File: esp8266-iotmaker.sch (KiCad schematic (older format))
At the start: 49 parts, among them J1 CONN_01X10, J2 CONN_01X10, Q1 S8050, Q2 S8050, SW1 SW_Push, SW2 SW_Push, U1 usb_mini_b, U2 chip-esp8266, U3 CP2102, U4 25Q32, U6 AMS1117-3.3, Y1 26MHz

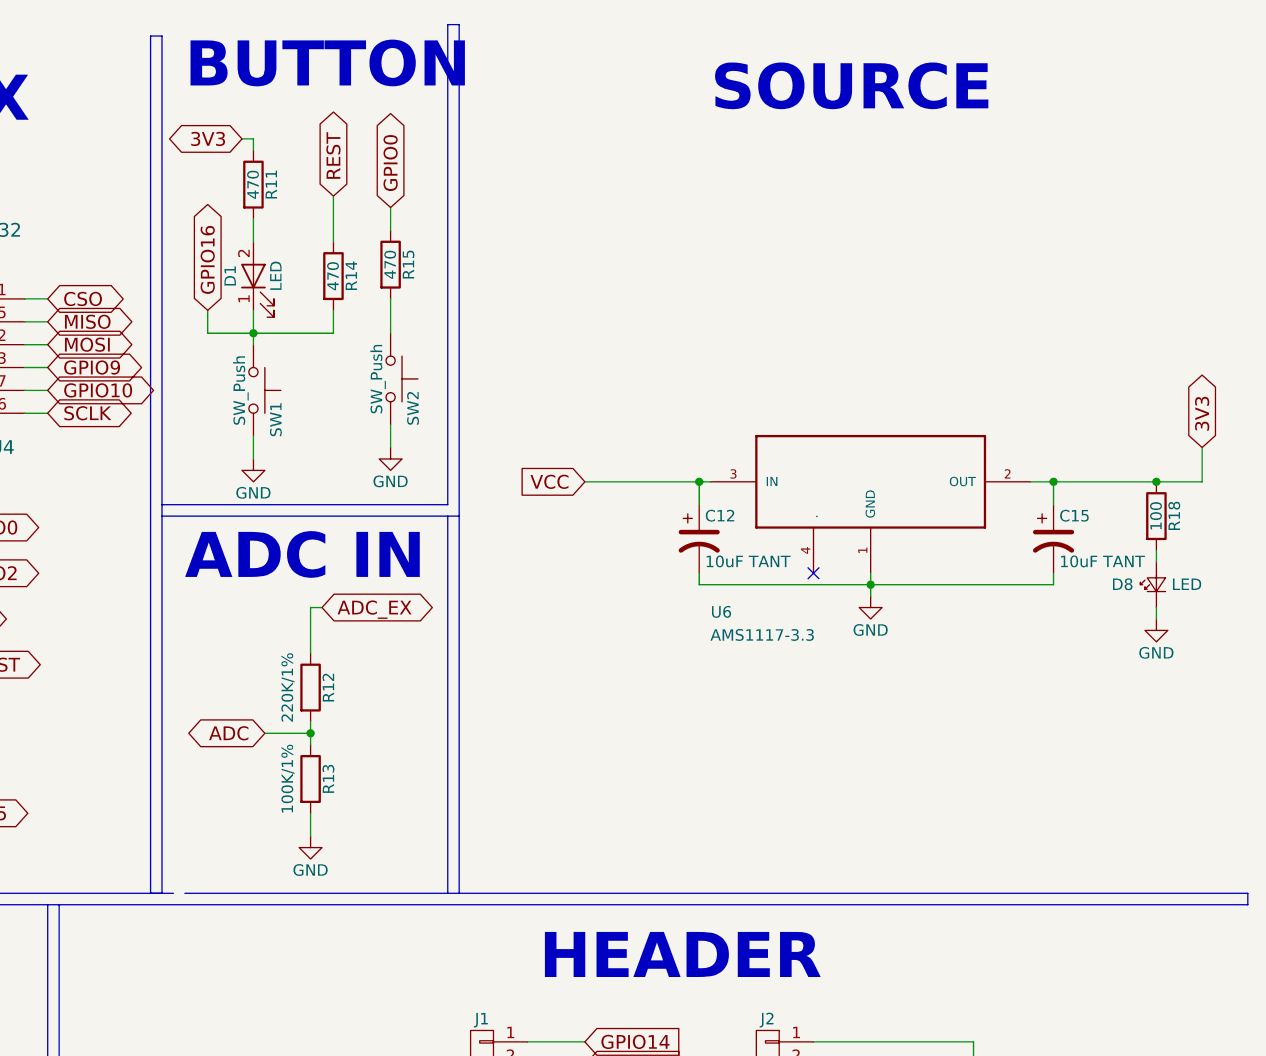
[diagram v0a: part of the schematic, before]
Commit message: edit solder mark
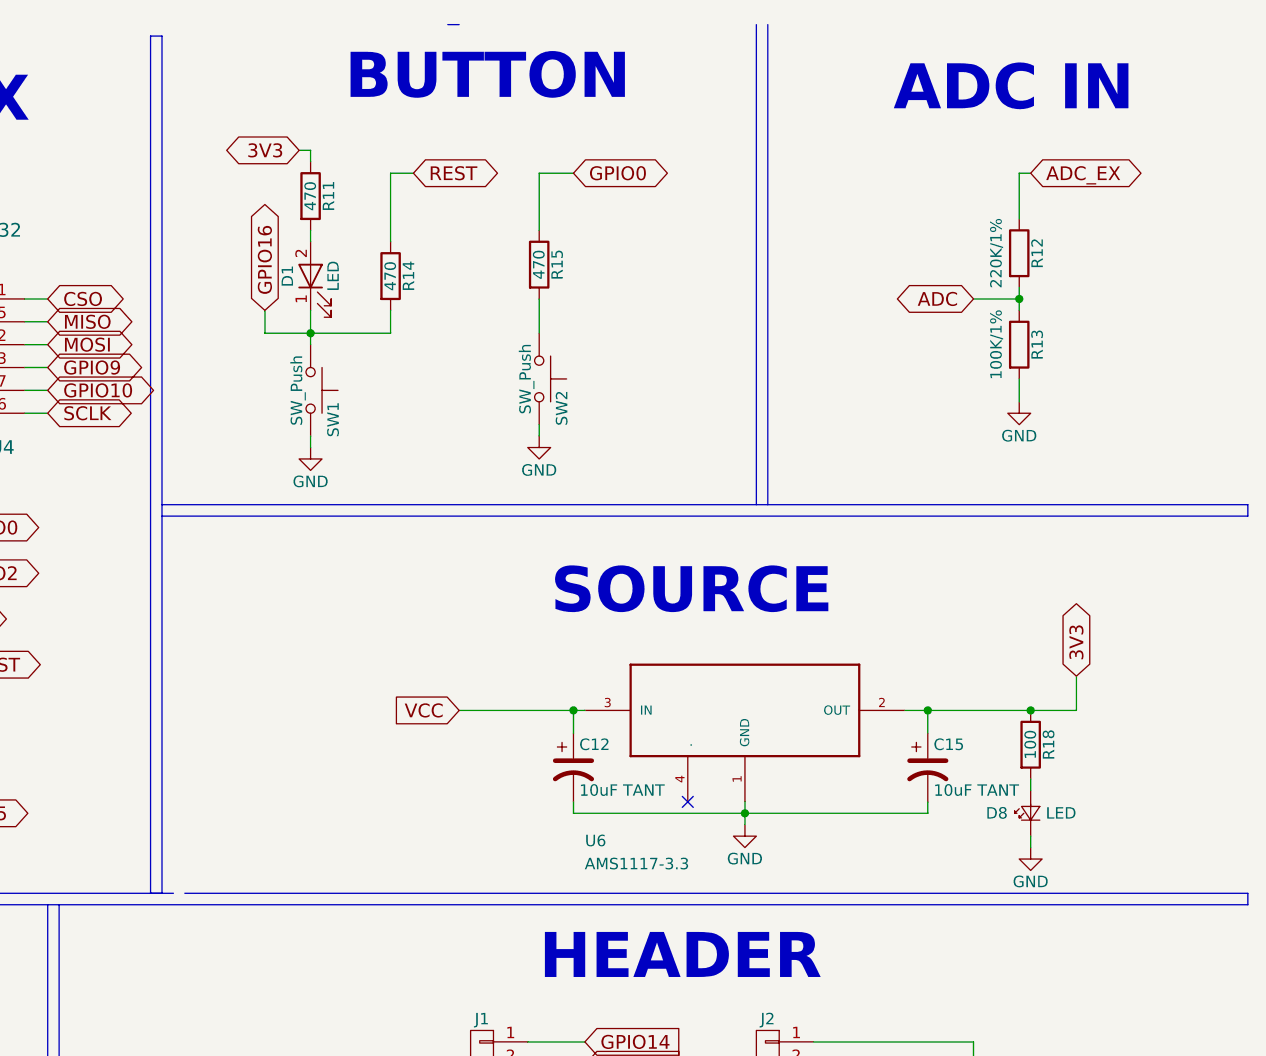
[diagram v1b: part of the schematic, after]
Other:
- moved on the sheet: C12, C15, D1, D8, R11, R12, R13, R14, R15, R18, SW1, SW2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

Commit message: edit readme
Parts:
- Y1: footprint Crystals:Crystal_SMD_2016-4pin_2.0x1.6mm -> Crystals:Crystal_SMD_5032-4pin_5.0x3.2mm
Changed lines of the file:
@@
 F 0 "Y1" H 3225 1150 50  0000 L CNN
 F 1 "26MHz" H 3225 1075 50  0000 L CNN
-F 2 "Crystals:Crystal_SMD_2016-4pin_2.0x1.6mm" H 3100 950 50  0001 C CNN
+F 2 "Crystals:Crystal_SMD_5032-4pin_5.0x3.2mm" H 3100 950 50  0001 C CNN
 F 3 "" H 3100 950 50  0001 C CNN
 	1    3100 950
